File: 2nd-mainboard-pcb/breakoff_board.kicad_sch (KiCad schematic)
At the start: 29 parts, among them J13 ISP, J14 Spannungsmessung, J7 Quartz

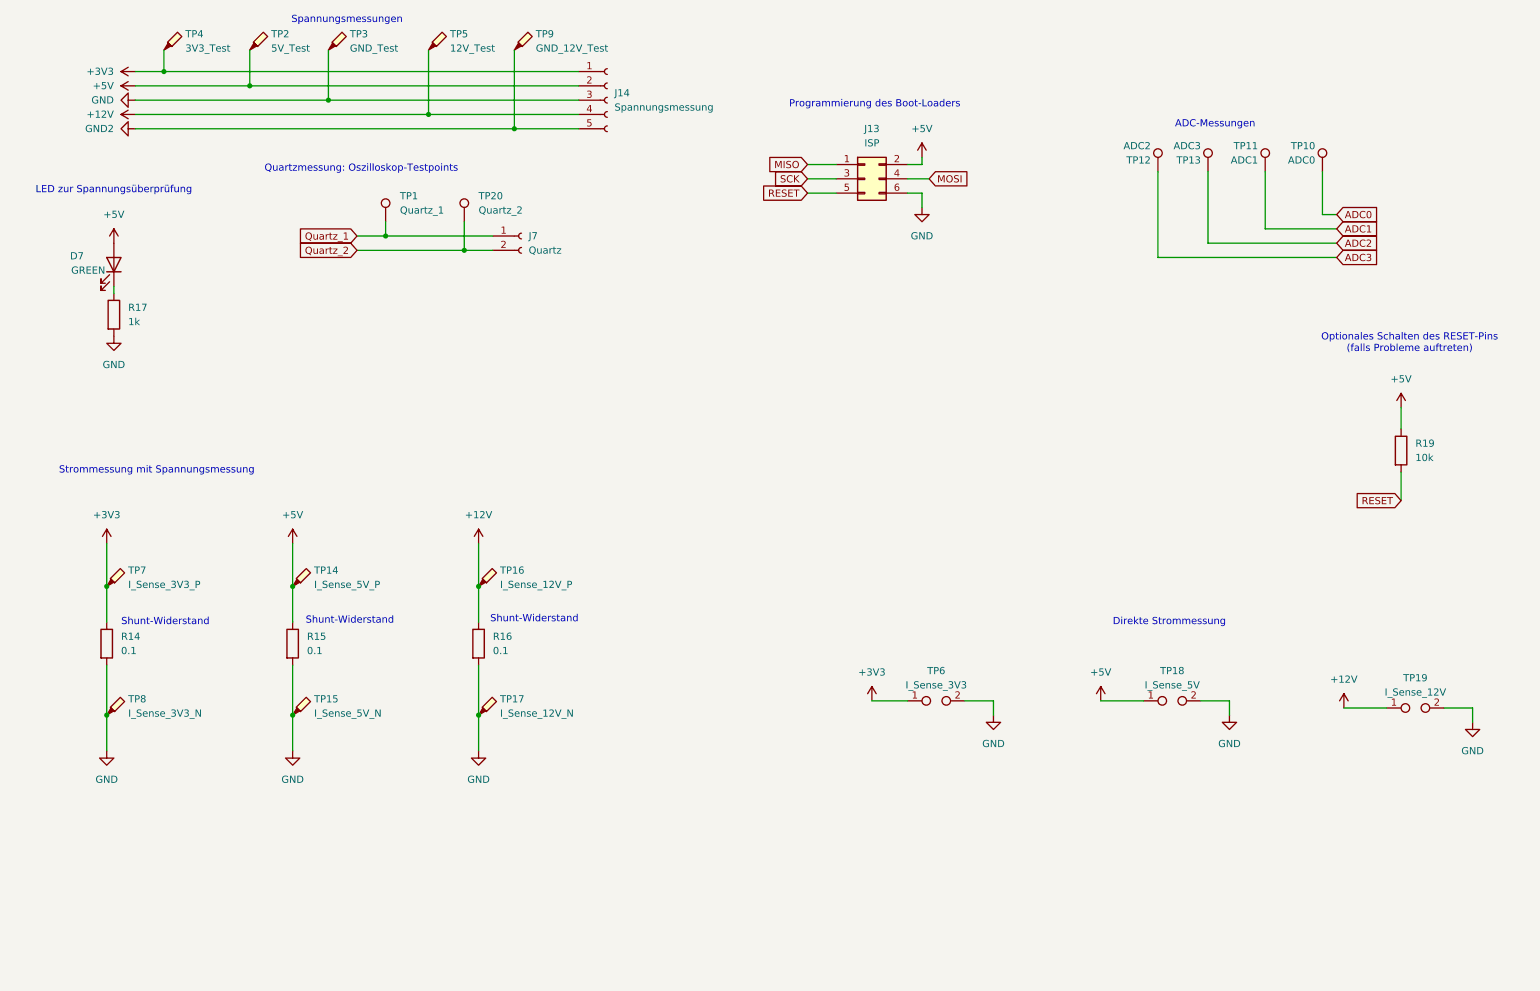
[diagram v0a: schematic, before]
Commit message: finished stacked design, annotaded
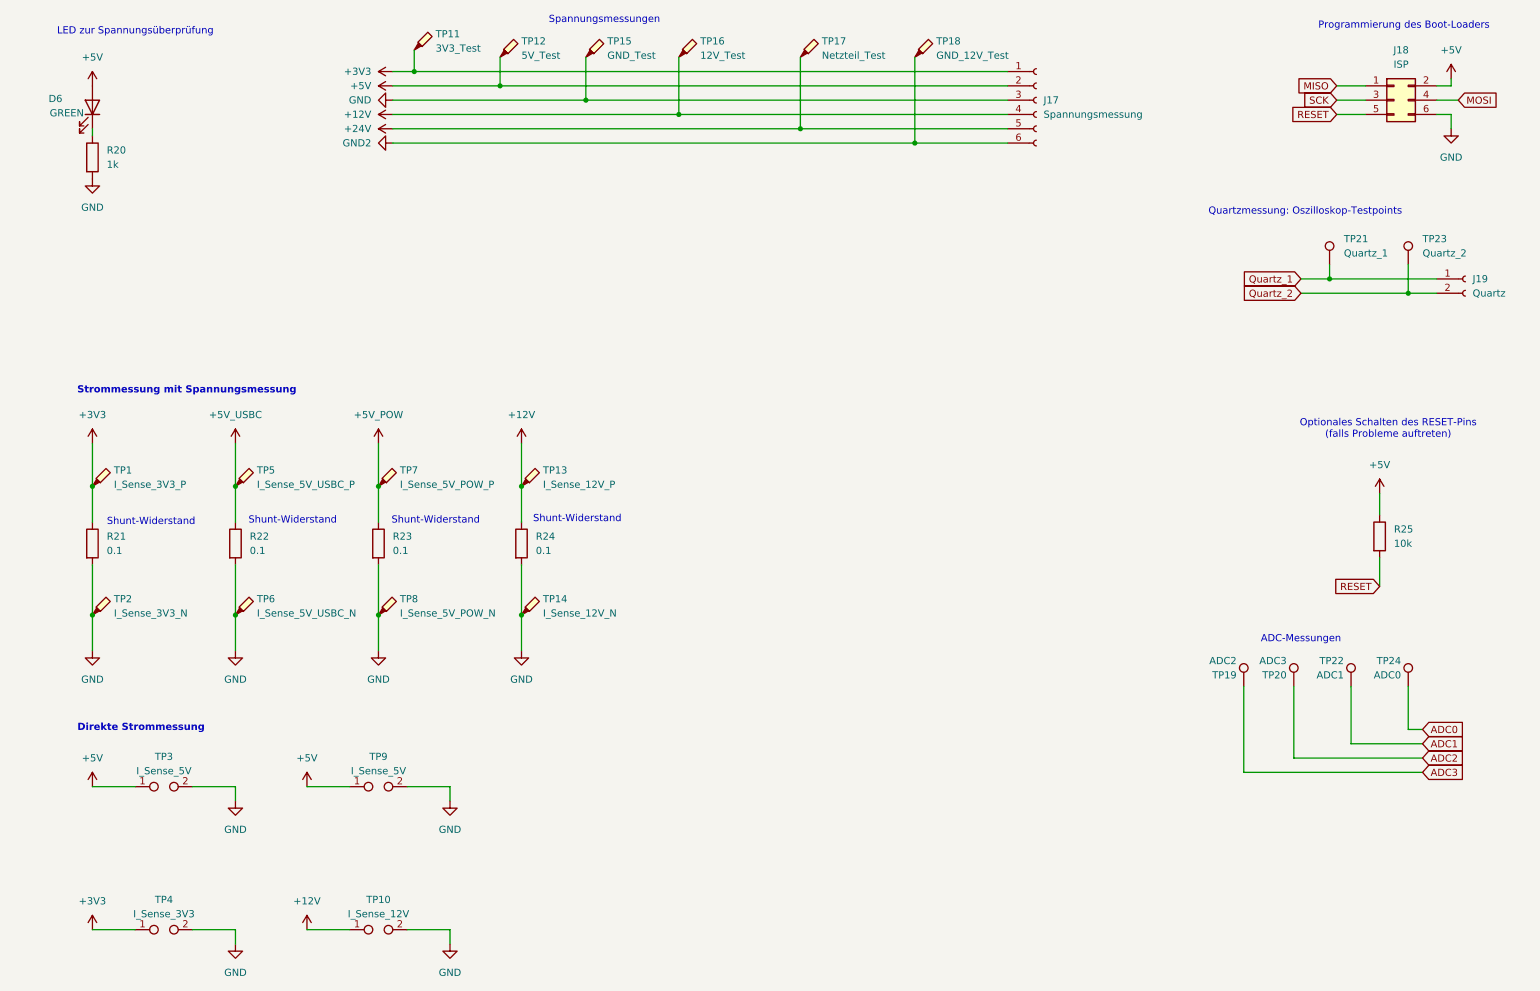
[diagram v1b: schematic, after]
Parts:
- removed J14: Spannungsmessung, symbol Connector:Conn_01x05_Socket
- removed R16: 0.1, symbol Device:R
- removed TP16: I_Sense_12V_P, symbol Connector:TestPoint_Probe
- added J17: Spannungsmessung, symbol Connector:Conn_01x06_Socket
- added R23, R24: 0.1, symbol Device:R
- added TP13: I_Sense_12V_P, symbol Connector:TestPoint_Probe
- added TP14: I_Sense_12V_N, symbol Connector:TestPoint_Probe
- added TP7: I_Sense_5V_POW_P, symbol Connector:TestPoint_Probe
- added TP8: I_Sense_5V_POW_N, symbol Connector:TestPoint_Probe
- added TP9: I_Sense_5V, symbol Connector:TestPoint_2Pole
- TP17: value I_Sense_12V_N -> Netzteil_Test; footprint (none) -> TestPoint:TestPoint_Pad_D3.0mm
- TP5: renamed from TP14; value I_Sense_5V_P -> I_Sense_5V_USBC_P
- TP6: renamed from TP15; value I_Sense_5V_N -> I_Sense_5V_USBC_N
- renumbered D7 to D6, J13 to J18, J7 to J19, R17 to R20, R14 to R21, R15 to R22, R19 to R25, TP7 to TP1, TP19 to TP10, TP4 to TP11, TP2 to TP12, TP3 to TP15, TP5 to TP16, TP9 to TP18, TP12 to TP19, TP8 to TP2, TP13 to TP20, TP1 to TP21, TP11 to TP22, TP20 to TP23, TP10 to TP24, TP18 to TP3, TP6 to TP4
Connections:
- net +12V: now also J17.4 (Pin_4), R24.1, TP13.1
- net +3V3: now also J17.1 (Pin_1)
- net +5V: now also J17.2 (Pin_2), TP9.1; no longer R22.1, TP5.1
- net GND: now also J17.3 (Pin_3), R23.2, R24.2, TP14.1, TP8.1, TP9.2; no longer TP17.1
- net GND2: now also J17.6 (Pin_6)
- new net +24V: J17.5 (Pin_5), TP17.1
- new net +5V_POW: R23.1, TP7.1
- new net +5V_USBC: R22.1, TP5.1
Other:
- moved on the sheet: D6, J18, J19, R20, R21, R22, R25, TP1, TP10, TP11, TP12, TP15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
